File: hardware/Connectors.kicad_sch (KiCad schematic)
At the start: 18 parts, among them J1 USB_C_Receptacle_USB2.0, J14 Conn_01x05, J2 M80-5302642, J3 M300-MV31045M1, J4 M80-5L10442MC, J5 M80-5L10442MC, J6 M80-5L10442MC

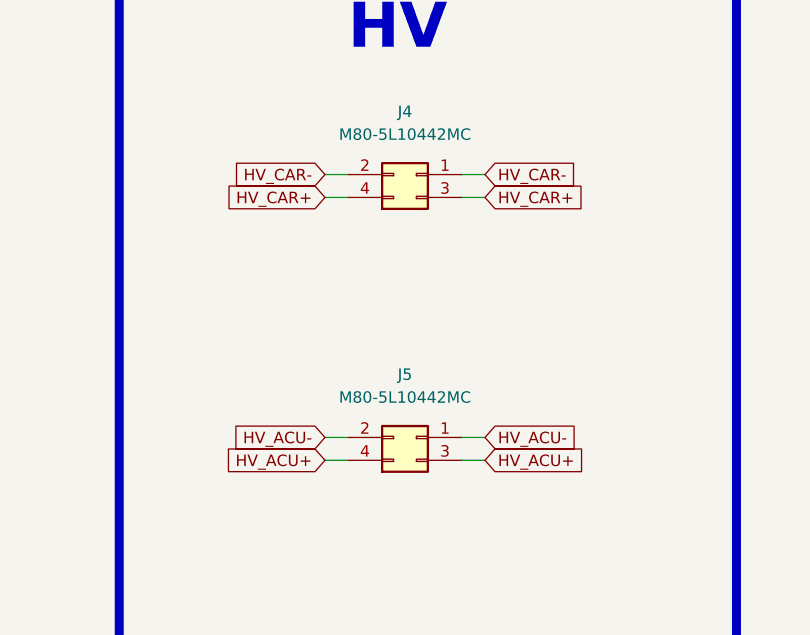
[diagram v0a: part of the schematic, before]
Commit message: board sync
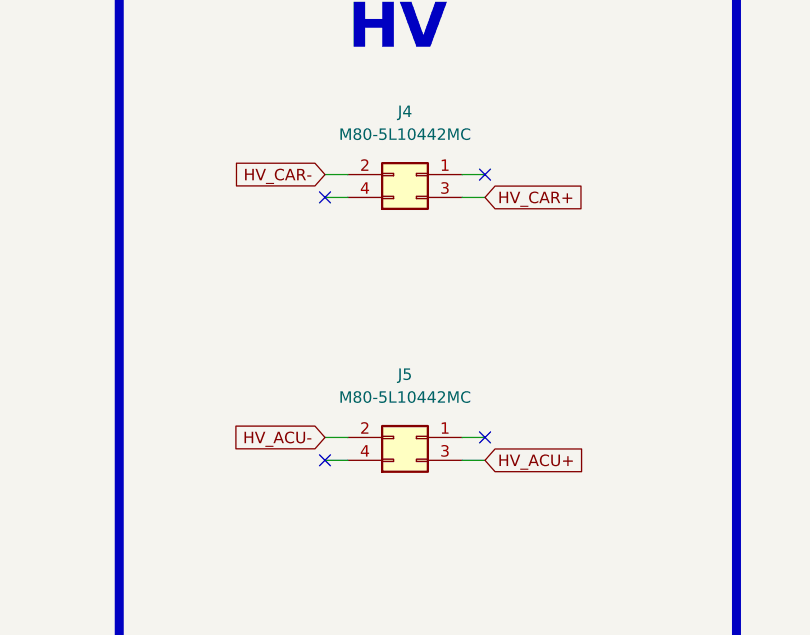
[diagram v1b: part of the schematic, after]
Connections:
- net HV_ACU+: no longer J5.4
- net HV_ACU-: no longer J5.1
- net HV_CAR+: no longer J4.4
- net HV_CAR-: no longer J4.1
- no-connect marks 2 -> 6
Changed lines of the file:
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@@
   (junction (at 121.92 136.525) (diameter 0) (color 0 0 0 0)
   )
+  (no_connect (at 187.96 41.275))
+  (no_connect (at 170.18 73.025))
+  (no_connect (at 170.18 43.815))
   (no_connect (at 263.525 66.675))
   (no_connect (at 263.525 69.215))
+  (no_connect (at 187.96 70.485))
   (wire (pts (xy 121.92 142.875) (xy 121.92 145.415))
     (stroke (width 0) (type default) (color 0 0 0 0))
@@
   )
   (wire (pts (xy 260.985 66.675) (xy 263.525 66.675))
-    (stroke (width 0) (type default) (color 0 0 0 0))
-  )
-  (wire (pts (xy 185.42 70.485) (xy 187.96 70.485))
     (stroke (width 0) (type default) (color 0 0 0 0))
   )
@@
     (stroke (width 0) (type default) (color 0 0 0 0))
   )
+  (wire (pts (xy 170.18 73.025) (xy 172.72 73.025))
+    (stroke (width 0) (type default) (color 0 0 0 0))
+  )
   (wire (pts (xy 268.605 43.815) (xy 268.605 46.355))
     (stroke (width 0) (type default) (color 0 0 0 0))
@@
   )
   (wire (pts (xy 81.915 80.01) (xy 79.375 80.01))
+    (stroke (width 0) (type default) (color 0 0 0 0))
+  )
+  (wire (pts (xy 185.42 70.485) (xy 187.96 70.485))
     (stroke (width 0) (type default) (color 0 0 0 0))
   )
@@
     (stroke (width 0) (type default) (color 0 0 0 0))
   )
-  (wire (pts (xy 172.72 73.025) (xy 170.18 73.025))
-    (stroke (width 0) (type default) (color 0 0 0 0))
-  )
   (wire (pts (xy 260.985 56.515) (xy 262.255 56.515))
     (stroke (width 0) (type default) (color 0 0 0 0))
@@
     )
   )
-  (global_label "HV_CAR+" (shape input) (at 170.18 43.815 180) (fields_autoplaced)
-    (effects (font (size 1.27 1.27)) (justify right))
-    (property "Intersheet References" "${INTERSHEET_REFS}" (id 0) (at 159.2682 43.7356 0)
-      (effects (font (size 1.27 1.27)) (justify right) hide)
-    )
-  )
   (global_label "IMD_SENSENSOR" (shape input) (at 53.975 97.155 180) (fields_autoplaced)
     (effects (font (size 1.27 1.27)) (justify right))
@@
     )
   )
-  (global_label "HV_ACU-" (shape input) (at 187.96 70.485 0) (fields_autoplaced)
-    (effects (font (size 1.27 1.27)) (justify left))
-    (property "Intersheet References" "${INTERSHEET_REFS}" (id 0) (at 198.9323 70.4056 0)
-      (effects (font (size 1.27 1.27)) (justify left) hide)
-    )
-  )
   (global_label "AIR_M_DETECTION" (shape input) (at 53.975 104.775 180) (fields_autoplaced)
     (effects (font (size 1.27 1.27)) (justify right))
@@
     )
   )
-  (global_label "HV_CAR-" (shape input) (at 187.96 41.275 0) (fields_autoplaced)
-    (effects (font (size 1.27 1.27)) (justify left))
-    (property "Intersheet References" "${INTERSHEET_REFS}" (id 0) (at 198.8718 41.1956 0)
-      (effects (font (size 1.27 1.27)) (justify left) hide)
-    )
-  )
   (global_label "D-" (shape input) (at 238.125 130.81 180) (fields_autoplaced)
     (effects (font (size 1.27 1.27)) (justify right))
@@
       (effects (font (size 1.27 1.27)) (justify right) hide)
     )
-  )
-  (global_label "HV_ACU+" (shape input) (at 170.18 73.025 180) (fields_autoplaced)
-    (effects (font (size 1.27 1.27)) (justify right))
-    (property "Intersheet References" "${INTERSHEET_REFS}" (id 0) (at 159.2077 72.9456 0)
-      (effects (font (size 1.27 1.27)) (justify right) hide)
-    )

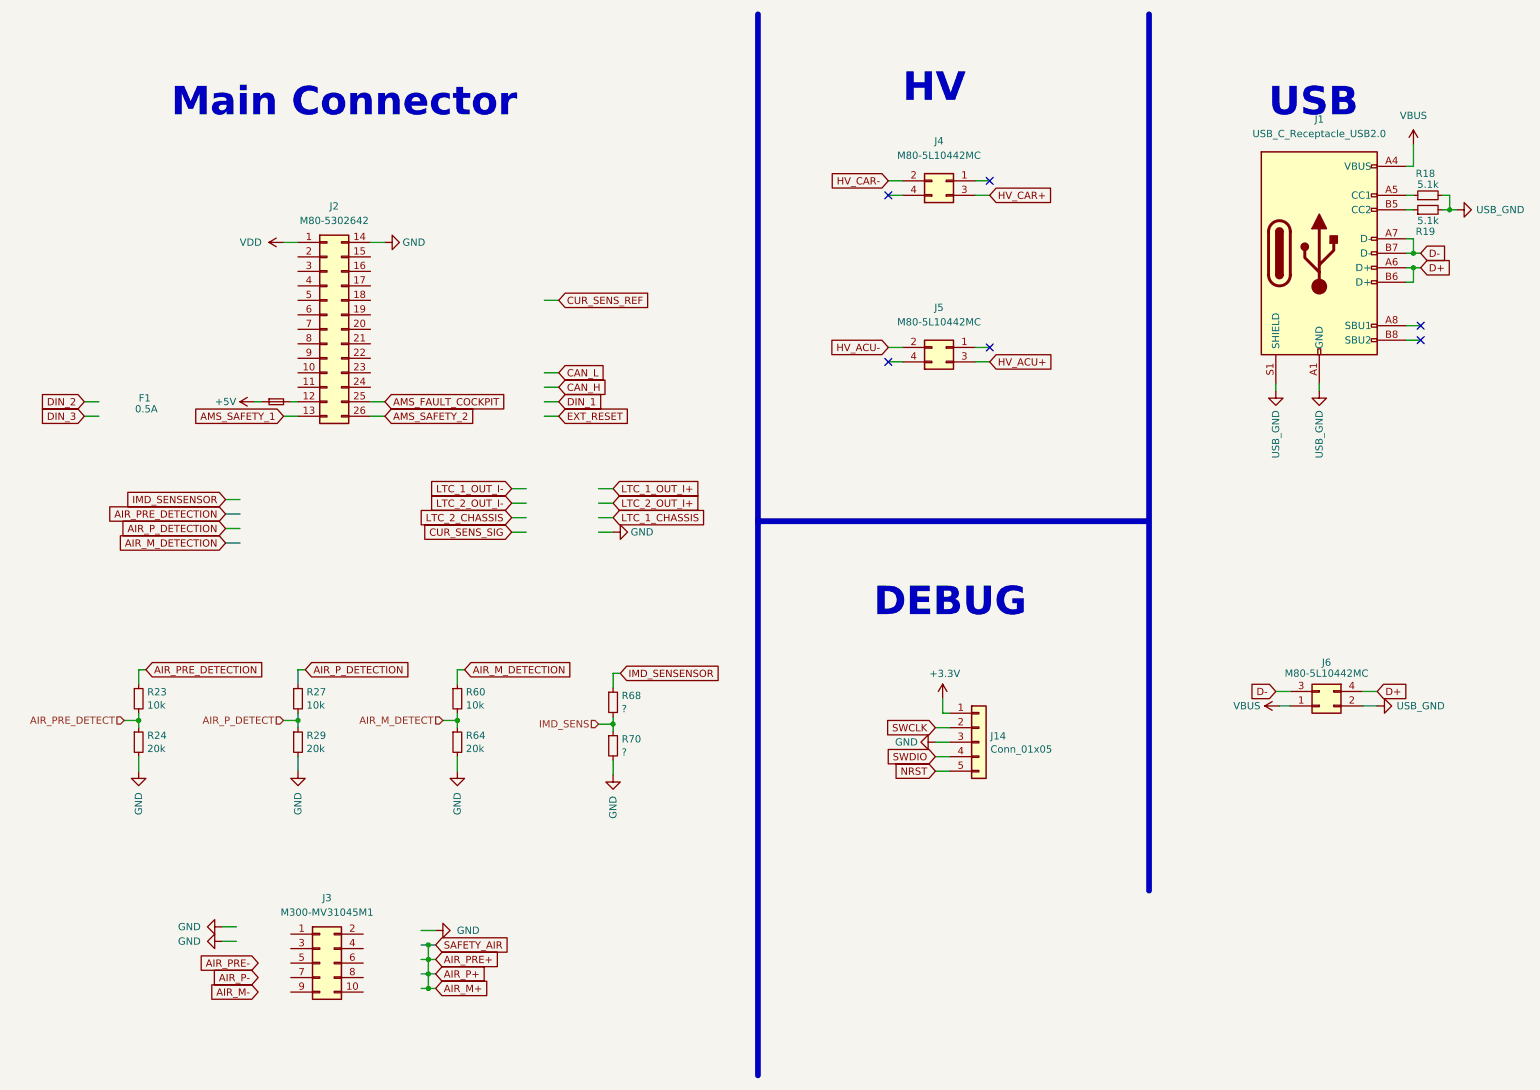
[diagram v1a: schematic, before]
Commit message: pcb iter 4?
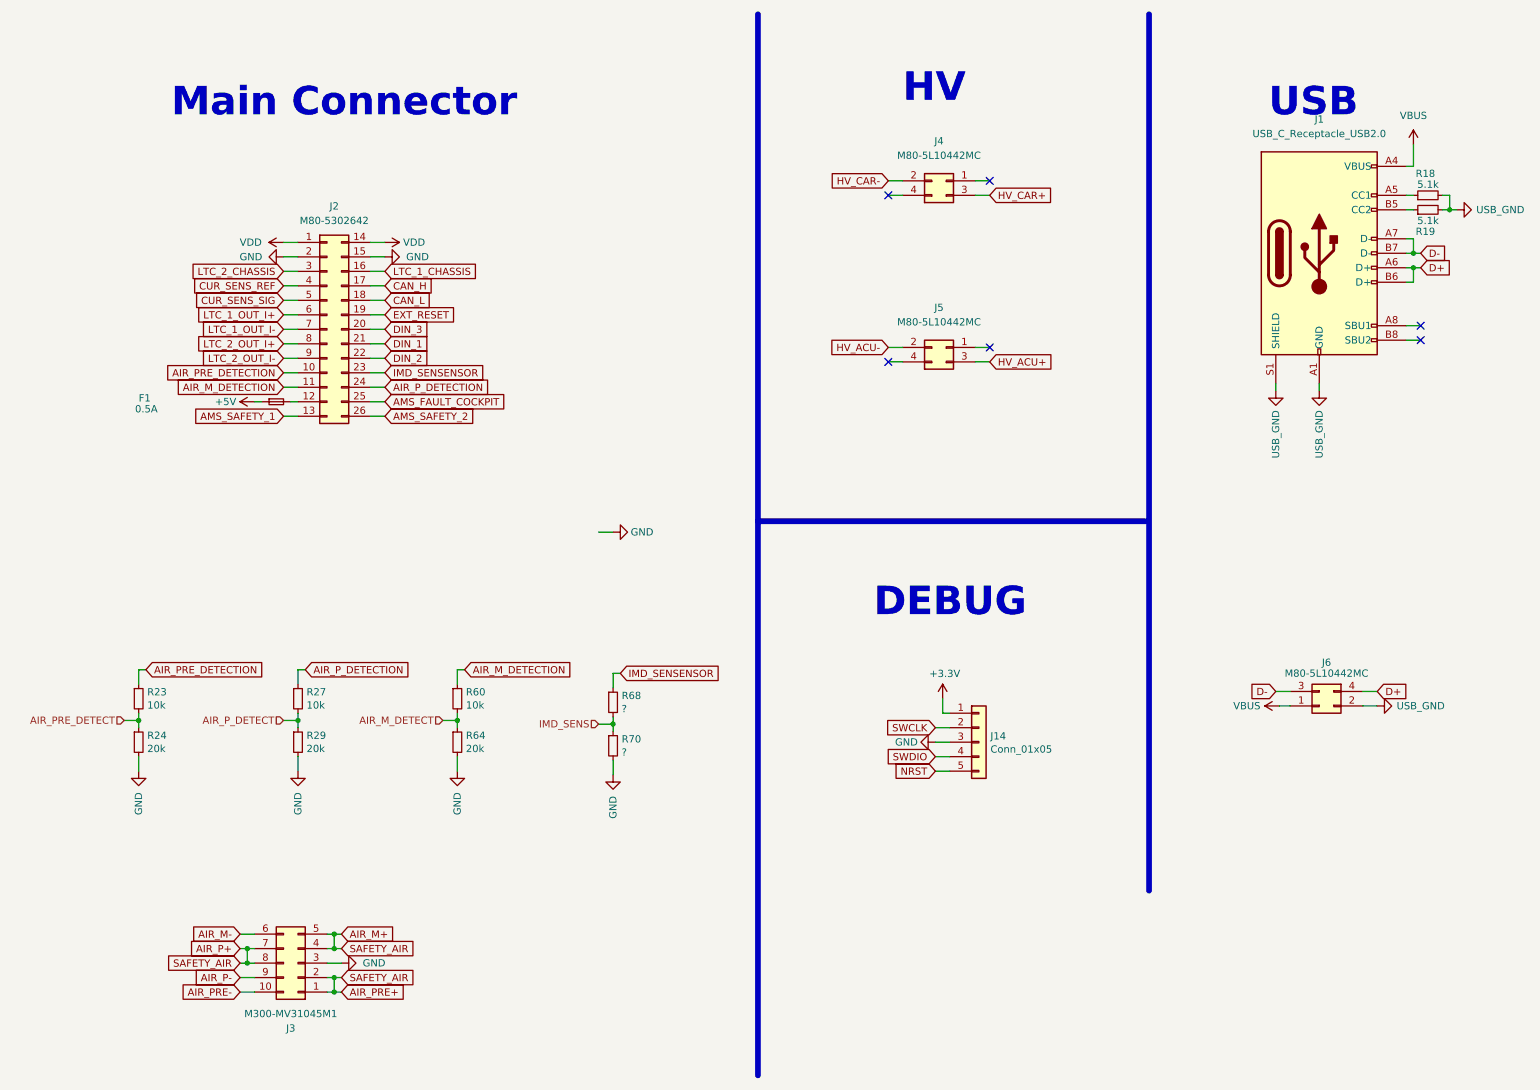
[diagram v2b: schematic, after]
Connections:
- net AIR_M+: now also J3.1, J3.2, J3.4, J3.5, J3.7, J3.8
- net AIR_M-: now also J3.6
- net AIR_M_DETECTION: now also J2.11
- net AIR_P-: now also J3.9
- net AIR_PRE-: now also J3.10
- net AIR_PRE_DETECTION: now also J2.10
- net AIR_P_DETECTION: now also J2.24
- net CAN_H: now also J2.17
- net CAN_L: now also J2.18
- net CUR_SENS_REF: now also J2.4
- net CUR_SENS_SIG: now also J2.5
- net DIN_1: now also J2.21
- net DIN_2: now also J2.22
- net DIN_3: now also J2.20
- net EXT_RESET: now also J2.19
- net GND: now also J2.15, J2.2, J3.3; no longer J2.14
- net IMD_SENSENSOR: now also J2.23
- net LTC_1_CHASSIS: now also J2.16
- net LTC_1_OUT_I+: now also J2.6
- net LTC_1_OUT_I-: now also J2.7
- net LTC_2_CHASSIS: now also J2.3
- net LTC_2_OUT_I+: now also J2.8
- net LTC_2_OUT_I-: now also J2.9
- net VDD: now also J2.14
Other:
- moved on the sheet: J3
